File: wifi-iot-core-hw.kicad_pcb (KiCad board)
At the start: 2 copper layers, 33 x 58.4 mm, 51 parts, among them P1 USB, P10 CONN_01X01, P11 CONN_01X01, P2 CONN_01X20, P3 CONN_01X20, P4 CONN_01X04, P8 CONN_01X01, P9 CONN_01X01, U1 LP2985LV, U2 STM32F103C8Tx, U3 ESP-07v2, Y1 8MHz, Y2 32.687

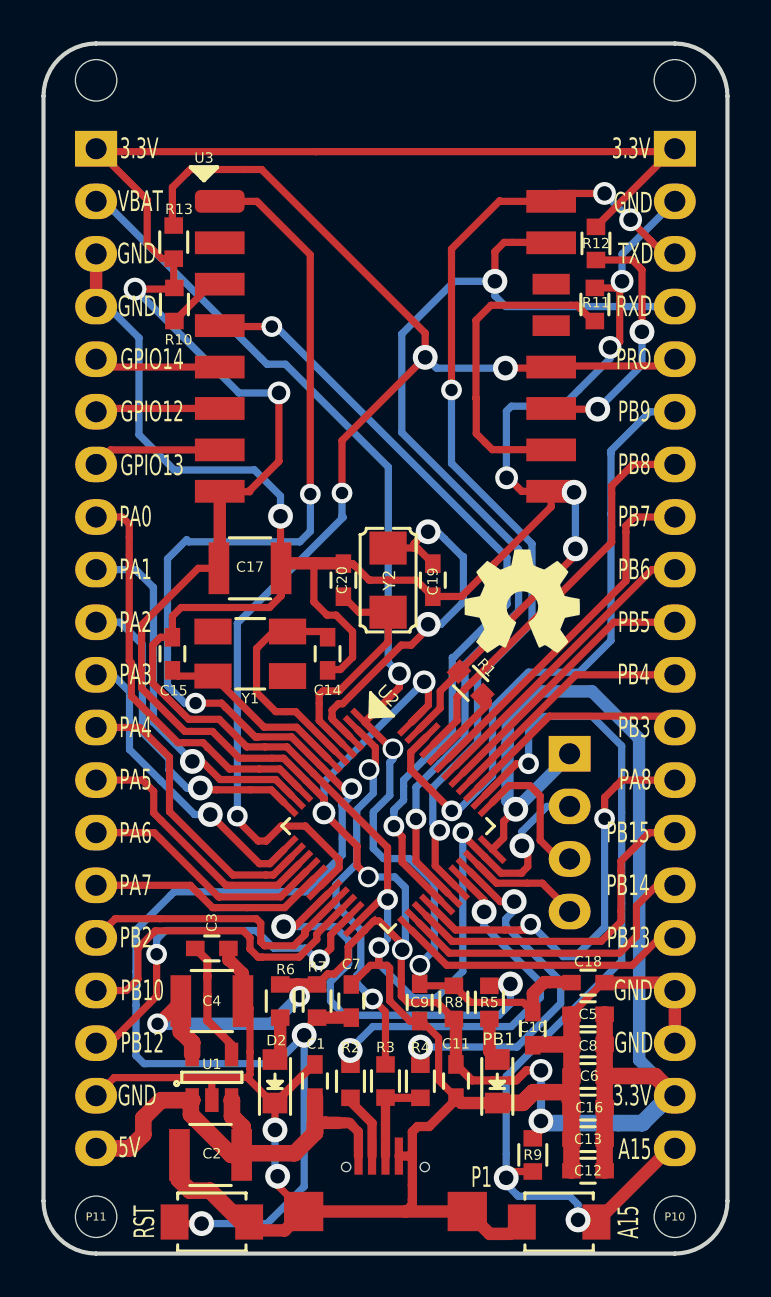
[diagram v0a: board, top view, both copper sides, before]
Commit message: Fix schematic & PCB
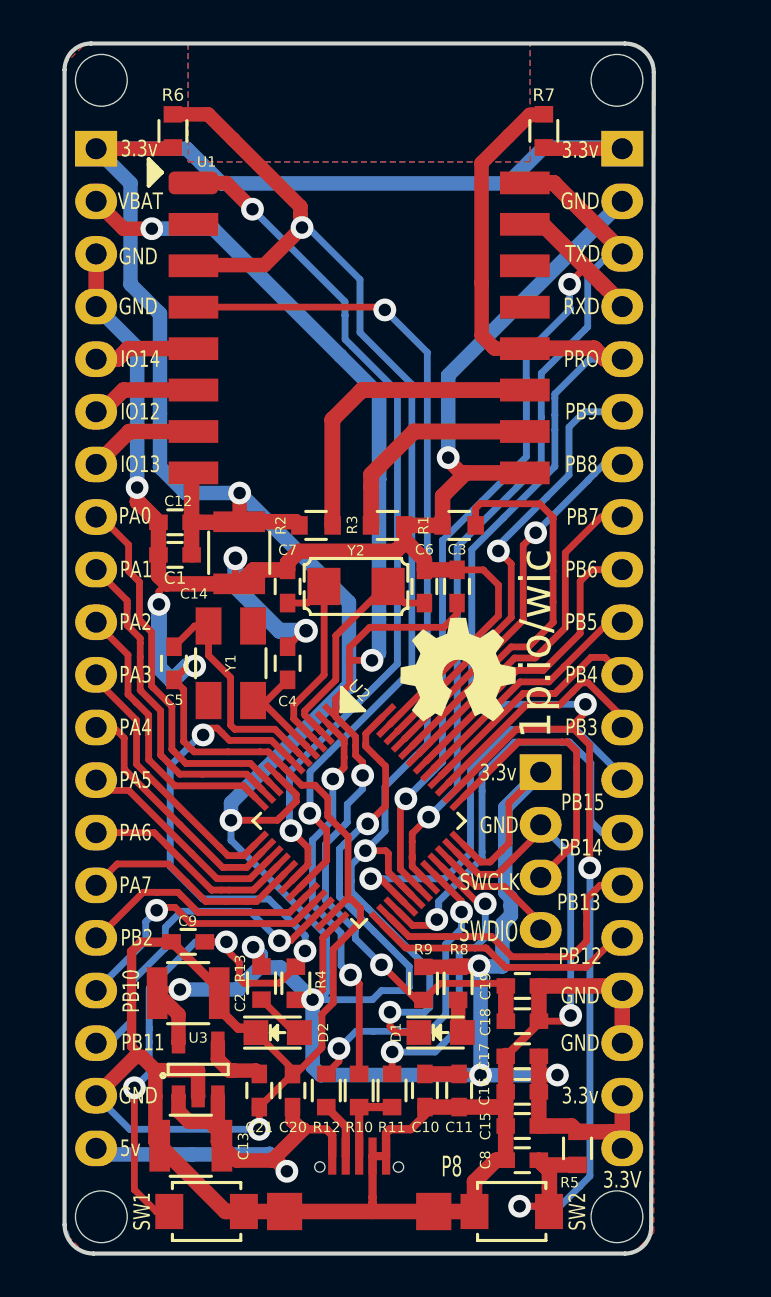
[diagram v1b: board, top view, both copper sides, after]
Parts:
- removed A15: SW_PUSH_SMALL_H, lib:SW_SPST_B3U-1000P-B
- removed P10, P11, P9: CONN_01X01, lib:MountingHole_2mm
- removed PB1: Led PWR, LEDs:LED_0805
- removed RST: RST, lib:SW_SPST_B3U-1000P-B
- added C21: 10nF, lib:C_0603, F.Cu at (117.1, 126.7)
- added D1: Led GPIO16, LEDs:LED_0805, F.Cu at (125.9, 123.9)
- added P5: CONN_01X01, lib:MountingHole_2.5mm, F.Cu at (109.5, 132.8)
- added P6: CONN_01X01, lib:MountingHole_2.5mm, F.Cu at (109.5, 78.0)
- added P7: CONN_01X04, Pin_Headers:Pin_Header_Straight_1x04, F.Cu at (130.7, 111.4)
- added SW1: RST, lib:SW_SPST_B3U-1000P-B, F.Cu at (114.6, 132.6)
- added SW2: SW_PUSH_SMALL_H, lib:SW_SPST_B3U-1000P-B, F.Cu at (129.3, 132.6)
- C13: value 0.1uF -> 10uF-50v; footprint lib:C_0603 -> Capacitors_SMD:C_1210
- C14: value 10pF -> 10uF-50v; footprint lib:C_0603 -> Capacitors_SMD:C_1210
- C15: value 10pF -> 0.1uF
- C16: value 0.1uF -> 1uF
- C17: value 10uF-50v -> 0.1uF; footprint Capacitors_SMD:C_1210 -> lib:C_0603
- C18: value 100nF -> 1uF
- C19: value 15pF -> 0.1uF
- C20: value 15pf -> 0.1uF
- C3: value 10nF -> 100nF
- C4: value 10uF-50v -> 10pF; footprint Capacitors_SMD:C_1210 -> lib:C_0603
- C5: value 0.1uF -> 10pF
- C6: value 1uF -> 15pF
- C7: value 0.1uF -> 15pf
- C8: value 0.1uF -> 470pF
- C9: value 1uF -> 0.1uF
- P1: value USB -> CONN_01X20; footprint lib:Micro_usb_B_smd -> Pin_Headers:Pin_Header_Straight_1x20
- P3: value CONN_01X20 -> CONN_01X01; footprint Pin_Headers:Pin_Header_Straight_1x20 -> lib:MountingHole_2.5mm
- P4: value CONN_01X04 -> CONN_01X01; footprint Pin_Headers:Pin_Header_Straight_1x04 -> lib:MountingHole_2.5mm
- P8: value CONN_01X01 -> USB; footprint lib:MountingHole_2mm -> lib:Micro_usb_B_smd
- R10: value 10K -> 1.5K
- R11, R12: value 10K -> 22
- R13, R7: value 10K -> 10k
- R2, R4: value 22 -> 10K
- R3: value 1.5K -> 10K
- R5: value 10k -> 10K
- R8: value 0R -> 10k
- R9: value 10K -> 0R
- U1: value LP2985LV -> ESP-07v2; footprint TO_SOT_Packages_SMD:SOT-23-5 -> lib:ESP-07v2-smd-16pin
- U3: value ESP-07v2 -> LP2985LV; footprint lib:ESP-07v2-smd-16pin -> TO_SOT_Packages_SMD:SOT-23-5
- moved P8 56.1 mm to (121.9, 132.6)
- moved P1 53.2 mm to (109.2, 81.3)
- moved R7 43.4 mm to (130.8, 80.4)
- moved U1 43.2 mm to (113.9, 82.9), turned to 0 degrees
- moved R12 42.9 mm to (120.3, 126.7)
- moved R6 42.3 mm to (112.9, 80.4), turned to 90 degrees
- moved U3 41.9 mm to (114.1, 125.7), turned to 90 degrees
- moved R11 39.2 mm to (123.5, 126.7), turned to 270 degrees
- moved R10 39.0 mm to (121.9, 126.7), turned to 270 degrees
- moved C12 37.1 mm to (113.0, 99.3), turned to 180 degrees
- moved R13 36.0 mm to (117.2, 121.6), turned to 270 degrees
- moved C15 28.4 mm to (129.8, 128.5), turned to 0 degrees
- moved C17 27.0 mm to (129.8, 125.1)
- moved R2 26.9 mm to (119.8, 99.5), turned to 0 degrees
- moved R3 26.8 mm to (123.3, 99.5), turned to 0 degrees
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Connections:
- C1 pad 1: +5V -> +3V3
- C10 pad 2: /VBAT -> +3V3
- C12 pad 1: GNDREF -> +3V3
- C12 pad 2: +3V3 -> GNDREF
- C13 pad 1: +3V3 -> +5V
- C14 pad 1: Net-(C14-Pad1) -> +3V3
- C15 pad 1: Net-(C15-Pad1) -> GNDREF
- C15 pad 2: GNDREF -> +3V3
- C16 pad 1: +3V3 -> GNDREF
- C16 pad 2: GNDREF -> +3V3
- C17 pad 1: +3V3 -> GNDREF
- C17 pad 2: GNDREF -> +3V3
- C19 pad 1: Net-(C19-Pad1) -> GNDREF
- C19 pad 2: GNDREF -> /VBAT
- C2 pad 1: +5V -> +3V3
- C20 pad 1: Net-(C20-Pad1) -> +5V
- C3 pad 1: Net-(C3-Pad1) -> GNDREF
- C3 pad 2: GNDREF -> /VBAT
- C4 pad 1: +3V3 -> Net-(C4-Pad1)
- C5 pad 1: GNDREF -> Net-(C5-Pad1)
- C5 pad 2: +3V3 -> GNDREF
- C6 pad 1: GNDREF -> Net-(C6-Pad1)
- C6 pad 2: +3V3 -> GNDREF
- C7 pad 1: /NRST -> Net-(C7-Pad1)
- C8 pad 1: GNDREF -> /ESP_PRO
- C8 pad 2: +3V3 -> GNDREF
- C9 pad 1: GNDREF -> /RST
- C9 pad 2: /VBAT -> GNDREF
- P1 pad 1: +5V -> +3V3
- P1 pad 2: Net-(P1-Pad2) -> /VBAT
- P1 pad 3: Net-(P1-Pad3) -> GNDREF
- P1 pad 5: GNDREF -> GPIO14
- P2 pad 10: PA2 -> PB5
- P2 pad 11: PA3 -> PB4
- P2 pad 12: PA4 -> PB3
- P2 pad 13: PA5 -> PB15
- P2 pad 14: PA6 -> PB14
- P2 pad 15: PA7 -> PB13
- P2 pad 16: PB2 -> PB12
- P2 pad 17: PB10 -> GNDREF
- P2 pad 18: PB11 -> GNDREF
- P2 pad 19: GNDREF -> +3V3
- P2 pad 2: /VBAT -> GNDREF
- P2 pad 20: +5V -> +3V3
- P2 pad 3: GNDREF -> /ESP_TXD
- P2 pad 4: GNDREF -> /ESP_RXD
- P2 pad 5: GPIO14 -> /ESP_PRO
- P2 pad 6: GPIO12 -> PB9
- P2 pad 7: GPIO13 -> PB8
- P2 pad 8: PA0 -> PB7
- P2 pad 9: PA1 -> PB6
- R10 pad 1: Net-(R10-Pad1) -> /USB_DIS
- R10 pad 2: +3V3 -> Net-(P8-Pad3)
- R11 pad 1: Net-(R11-Pad1) -> /USB_DP
- R11 pad 2: GNDREF -> Net-(P8-Pad3)
- R12 pad 1: +3V3 -> /USB_DM
- R12 pad 2: Net-(R12-Pad2) -> Net-(P8-Pad2)
- R13 pad 2: /PRO -> Net-(D2-Pad2)
- R2 pad 1: /USB_DM -> +3V3
- R2 pad 2: Net-(P1-Pad2) -> Net-(R2-Pad2)
- R3 pad 1: /USB_DIS -> Net-(R3-Pad1)
- R3 pad 2: Net-(P1-Pad3) -> GNDREF
- R4 pad 1: /USB_DP -> /RST
- R4 pad 2: Net-(P1-Pad3) -> +3V3
- R5 pad 1: Led_u -> /ESP_PRO
- R5 pad 2: Net-(D1-Pad2) -> +3V3
- R6 pad 2: Net-(D2-Pad2) -> /CH_PD
- R7 pad 1: /NRST -> +3V3
- R7 pad 2: +3V3 -> /ESP_PRO
- R8 pad 1: /VBAT -> +3V3
- R8 pad 2: +3V3 -> Net-(D1-Pad2)
- R9 pad 1: /BUTTON -> /VBAT
- U1 pad 1: +5V -> /ESP_RST
- U1 pad 2: GNDREF -> Net-(U1-Pad2)
- U1 pad 3: +5V -> /CH_PD
- U1 pad 4: Net-(C3-Pad1) -> /GPIO16
- U1 pad 5: +3V3 -> GPIO14
- U2 pad 18: /PRO -> /ESP_RST
- U2 pad 19: Led_u -> /CH_PD
- U2 pad 29: GPIO16 -> /GPIO16
- U2 pad 3: Net-(C19-Pad1) -> Net-(C6-Pad1)
- U2 pad 38: /BUTTON -> /ESP_PRO
- U2 pad 4: Net-(C20-Pad1) -> Net-(C7-Pad1)
- U2 pad 5: Net-(C14-Pad1) -> Net-(C4-Pad1)
- U2 pad 6: Net-(C15-Pad1) -> Net-(C5-Pad1)
- U2 pad 7: /NRST -> /RST
- U3 pad 1: /NRST -> +5V
- U3 pad 2: Net-(U3-Pad2) -> GNDREF
- U3 pad 3: Net-(R10-Pad1) -> +5V
- U3 pad 4: GPIO16 -> Net-(C21-Pad1)
- U3 pad 5: GPIO14 -> +3V3
- Y1 pad 1: Net-(C14-Pad1) -> Net-(C4-Pad1)
- Y1 pad 2: Net-(C15-Pad1) -> Net-(C5-Pad1)
- Y2 pad 1: Net-(C19-Pad1) -> Net-(C6-Pad1)
- Y2 pad 2: Net-(C20-Pad1) -> Net-(C7-Pad1)
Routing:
- net /NRST: track 90.3 -> 0.00 mm, vias 5 -> 0
- net /ESP_PRO: track 0.00 -> 86.6 mm, vias 0 -> 3
- net /PRO: track 65.5 -> 0.00 mm, vias 4 -> 0
- net /GPIO16: track 0.00 -> 54.8 mm, vias 0 -> 3
- net /CH_PD: track 0.00 -> 52.3 mm, vias 0 -> 2
- net /RST: track 0.00 -> 45.6 mm, vias 0 -> 4
- net /BUTTON: track 45.4 -> 0.00 mm, vias 3 -> 0
- net /ESP_RST: track 0.00 -> 44.9 mm, vias 0 -> 2
- net GPIO16: track 38.4 -> 0.00 mm, vias 2 -> 0
- net /VBAT: track 57.6 -> 80.9 mm
- net Led_u: track 20.8 -> 0.00 mm, vias 2 -> 0
- net Net-(C19-Pad1): track 18.8 -> 0.00 mm, vias 2 -> 0
- net Net-(R11-Pad1): track 15.8 -> 0.00 mm
- net Net-(R1-Pad1): track 3.78 -> 19.3 mm
- net Net-(R2-Pad2): track 0.00 -> 15.0 mm
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- added copper zone on B.Cu, net GNDREF
- added copper zone on F.Cu, net GNDREF
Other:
- board size 33 x 58.4 mm -> 28.4 x 58.4 mm
- net class Default: trace_width 0.35 -> 0.33; via_dia 1 -> 1.1; via_drill 0.7 -> 0.6
- rule trace_min: 0.3 -> 0.33
- rule via_min_size: 1 -> 1.1
- board text added: "1p.io/wic"
- board text added: "3.3v"
- board text added: "5v"
- board text added: "IO12"
- board text added: "IO13"
- board text added: "IO14"
- board text added: "PB11"
- board text added: "SWCLK"
- board text added: "SWDIO"
- board text removed: "5V"
- board text removed: "A15"
- board text removed: "GPIO12"
- board text removed: "GPIO13"
- board text removed: "GPIO14"
- board text removed: "PA8"
